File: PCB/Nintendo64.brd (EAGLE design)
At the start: 73 x 29 mm, 15 parts, among them U1 ESP32DEVKITC

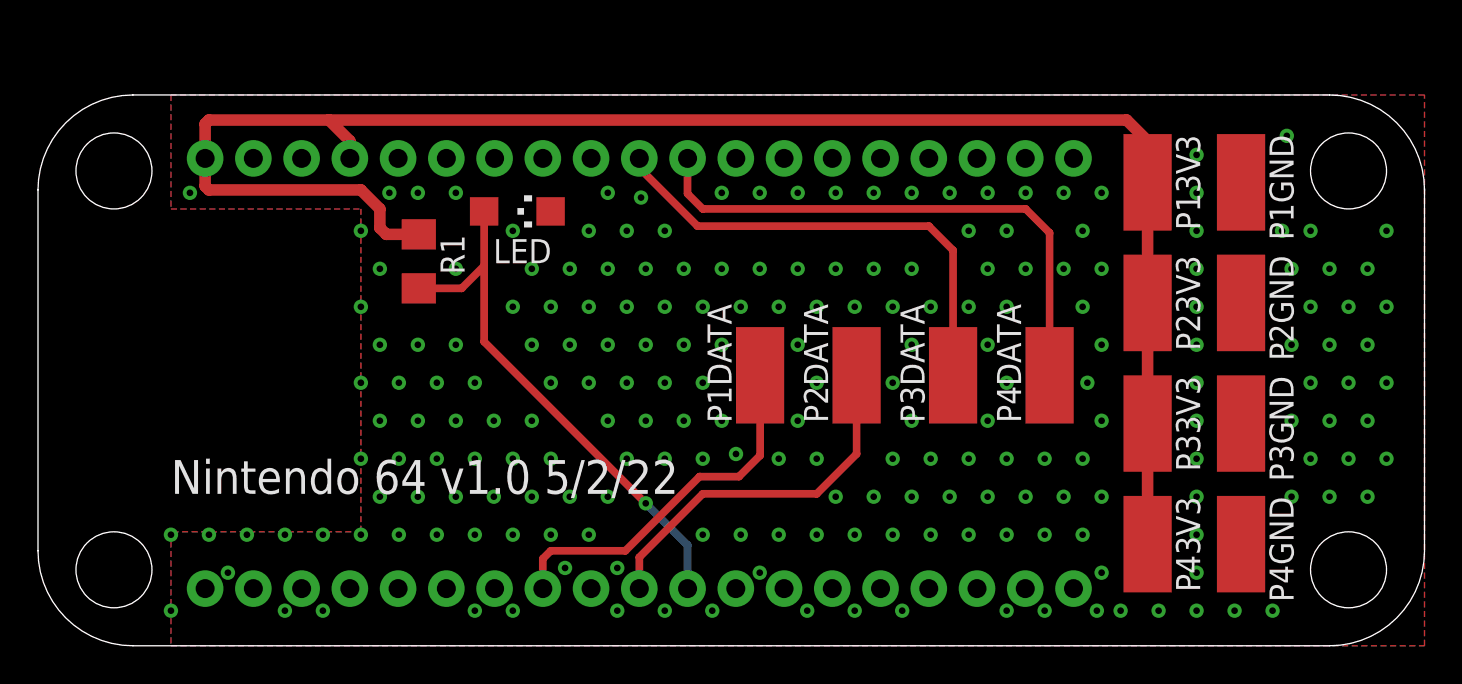
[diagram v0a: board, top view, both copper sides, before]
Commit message: Updated PCBs
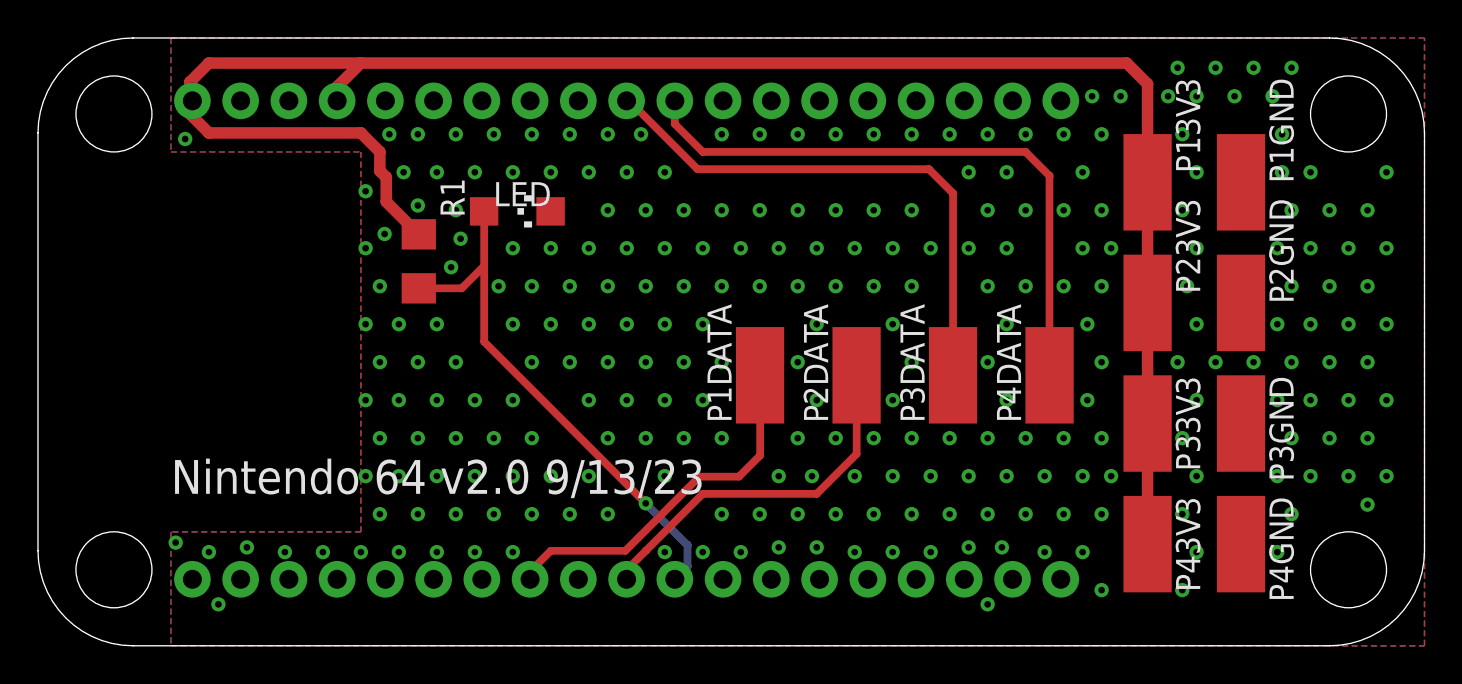
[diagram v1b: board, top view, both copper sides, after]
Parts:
- removed U1: ESP32DEVKITC, ESP32-DEVKITC:ESP32-DEVKITC
- added U2: ESP32DEVKITC, ESP32-DEVKITC4:ESP32-DEVKITC
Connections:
- net 3V3: now also U2.1, U2.4; no longer U1.1, U1.4
- net GND: now also U2.14, U2.32, U2.33, U2.36, U2.38, U2.5, U2.6, U2.7, U2.8, U2.9; no longer U1.14, U1.32, U1.33, U1.36, U1.38, U1.5, U1.6, U1.7, U1.8, U1.9
- net LED: now also U2.28; no longer U1.28
- net P1DATA: now also U2.31; no longer U1.31
- net P2DATA: now also U2.29; no longer U1.29
- net P3DATA: now also U2.10; no longer U1.10
- net P4DATA: now also U2.11; no longer U1.11
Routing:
- net 3V3: track 90.0 -> 95.9 mm
- net P3DATA: track 25.4 -> 28.8 mm
- net P4DATA: track 29.3 -> 32.6 mm
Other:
- board size 73 x 29 mm -> 73 x 32 mm
- board text added: "Nintendo 64 v2.0 9/13/23"
- board text removed: "Nintendo 64 v1.0 5/2/22"
